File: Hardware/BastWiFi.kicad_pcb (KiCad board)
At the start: 2 copper layers, 60 x 22.9 mm, 31 parts, among them J1 Conn_Battery, J3 Conn_Left, J4 Conn_Right, P1 USB_C_Plug_USB2.0, Q1 DMG3415U-7, SW1 GPIO0, SW2 RESET, U1 MCP73831-3-OT, U2 AP2112K-3.3, U3 ESP32-S2-WROVER

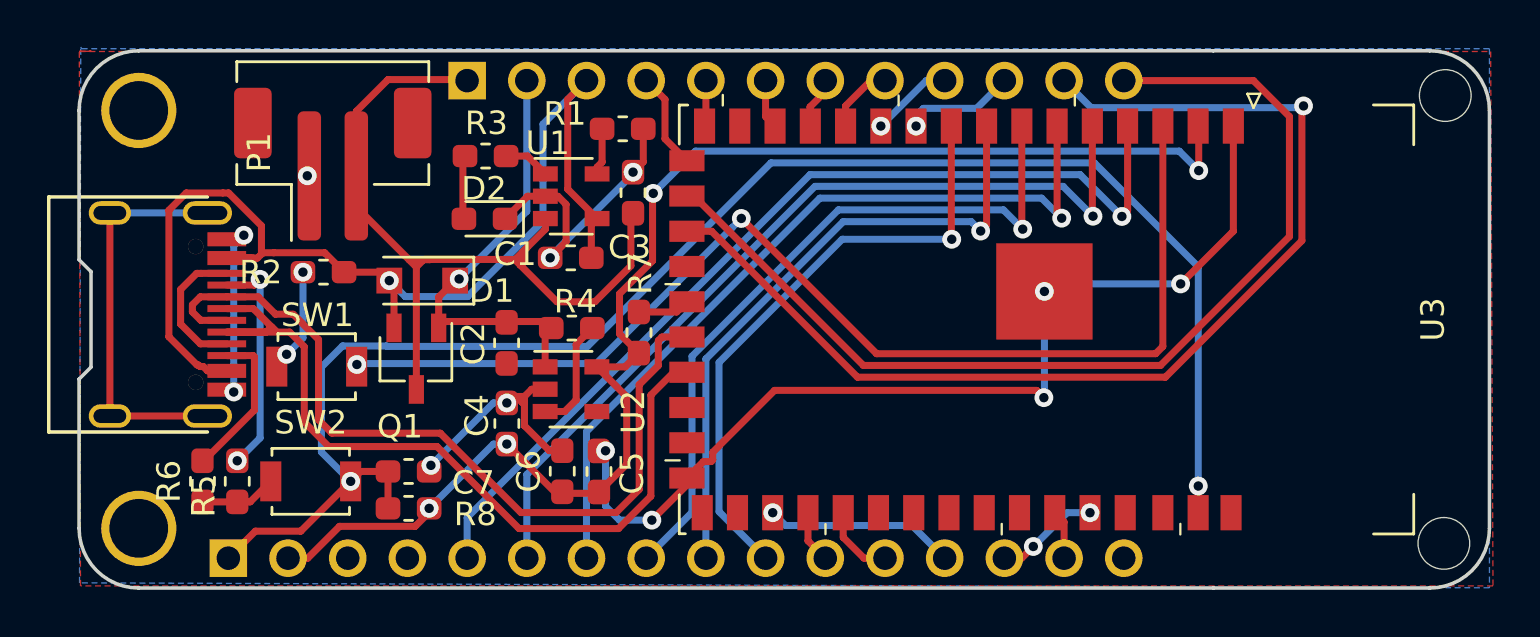
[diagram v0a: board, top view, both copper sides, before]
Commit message: Change tracks
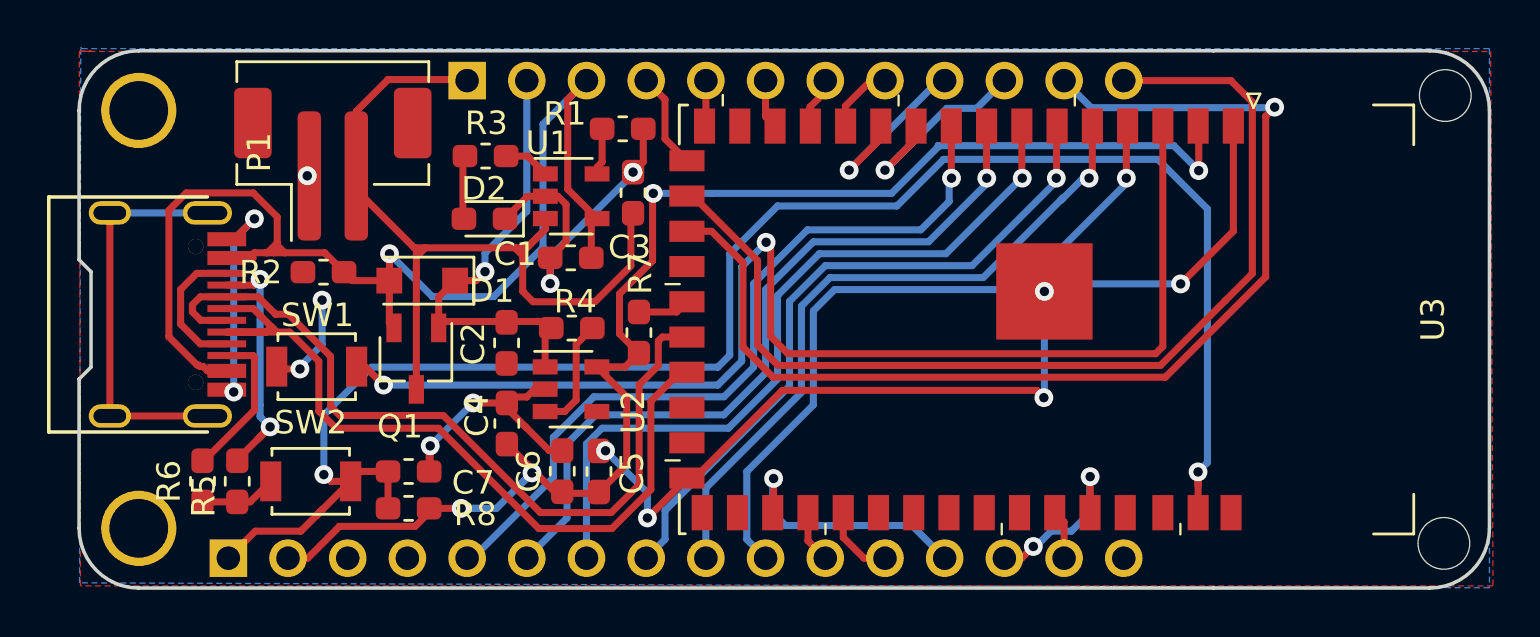
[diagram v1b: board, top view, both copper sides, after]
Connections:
- J3 pad 10: /A5 -> /A0
- J3 pad 5: /A0 -> /A5
- J3 pad 6: /A1 -> /A4
- J3 pad 7: /A2 -> /A3
- J3 pad 8: /A3 -> /A2
- J3 pad 9: /A4 -> /A1
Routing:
- net /A0: track 40.3 -> 30.1 mm
- net /A1: track 37.1 -> 29.7 mm
- net /A5: track 26.0 -> 33.1 mm
- net /A4: track 27.3 -> 32.6 mm
- net /~RST~: track 68.5 -> 73.5 mm
- net /A2: track 34.1 -> 29.3 mm
- net /GPIO06: track 3.52 -> 8.08 mm
- net VBUS: track 49.6 -> 54.2 mm
- net /GPIO05: track 4.82 -> 9.08 mm
- net /GPIO0: track 49.0 -> 53.0 mm
- net GND: track 81.6 -> 85.2 mm
- net /RX: track 4.44 -> 7.55 mm
- net /MISO: track 8.12 -> 11.1 mm
- net +3V3: track 58.5 -> 60.6 mm
- net /A3: track 30.8 -> 32.5 mm
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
